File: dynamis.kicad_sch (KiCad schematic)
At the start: 201 parts, among them J0 USB_C_Receptacle_USB2.0, SW00_00 SW_Push, SW00_01 SW_Push, SW00_02 SW_Push, SW00_03 SW_Push, SW00_04 SW_Push, SW00_05 SW_Push, SW00_06 SW_Push, SW01_00 SW_Push, SW01_01 SW_Push, SW01_02 SW_Push, SW01_03 SW_Push, SW01_04 SW_Push, SW01_05 SW_Push, SW01_06 SW_Push, SW02_01 SW_Push, SW02_02 SW_Push, SW02_03 SW_Push, SW02_04 SW_Push, SW02_05 SW_Push, SW02_06 SW_Push, SW03_00 SW_Push, SW03_02 SW_Push, SW03_03 SW_Push, SW03_04 SW_Push, SW03_05 SW_Push, SW03_06 SW_Push, SW04_00 SW_Push, SW04_01 SW_Push, SW04_02 SW_Push, SW04_03 SW_Push, SW04_05 SW_Push, SW04_06 SW_Push, SW05_01 SW_Push, SW05_02 SW_Push, SW05_03 SW_Push, SW05_04 SW_Push, SW05_05 SW_Push, SW05_06 SW_Push, SW06_00 SW_Push, SW06_01 SW_Push, SW06_02 SW_Push, SW06_03 SW_Push, SW06_04 SW_Push, SW06_05 SW_Push, SW06_06 SW_Push, SW07_01 SW_Push, SW07_02 SW_Push, SW07_03 SW_Push, SW07_04 SW_Push, SW07_05 SW_Push, SW07_06 SW_Push, SW08_00 SW_Push, SW08_02 SW_Push, SW08_03 SW_Push, SW08_04 SW_Push, SW08_05 SW_Push, SW08_06 SW_Push, SW09_00 SW_Push, SW09_01 SW_Push, SW09_02 SW_Push, SW09_03 SW_Push, SW09_04 SW_Push, SW09_05 SW_Push, SW09_06 SW_Push, U0 ATmega32U4-M, U1 PMW3360DM-T2QU, U2 TPS73601DBV, U3 TPS73601DBV, U4 TPD4E05U06DQAR, Y0 16Mhz

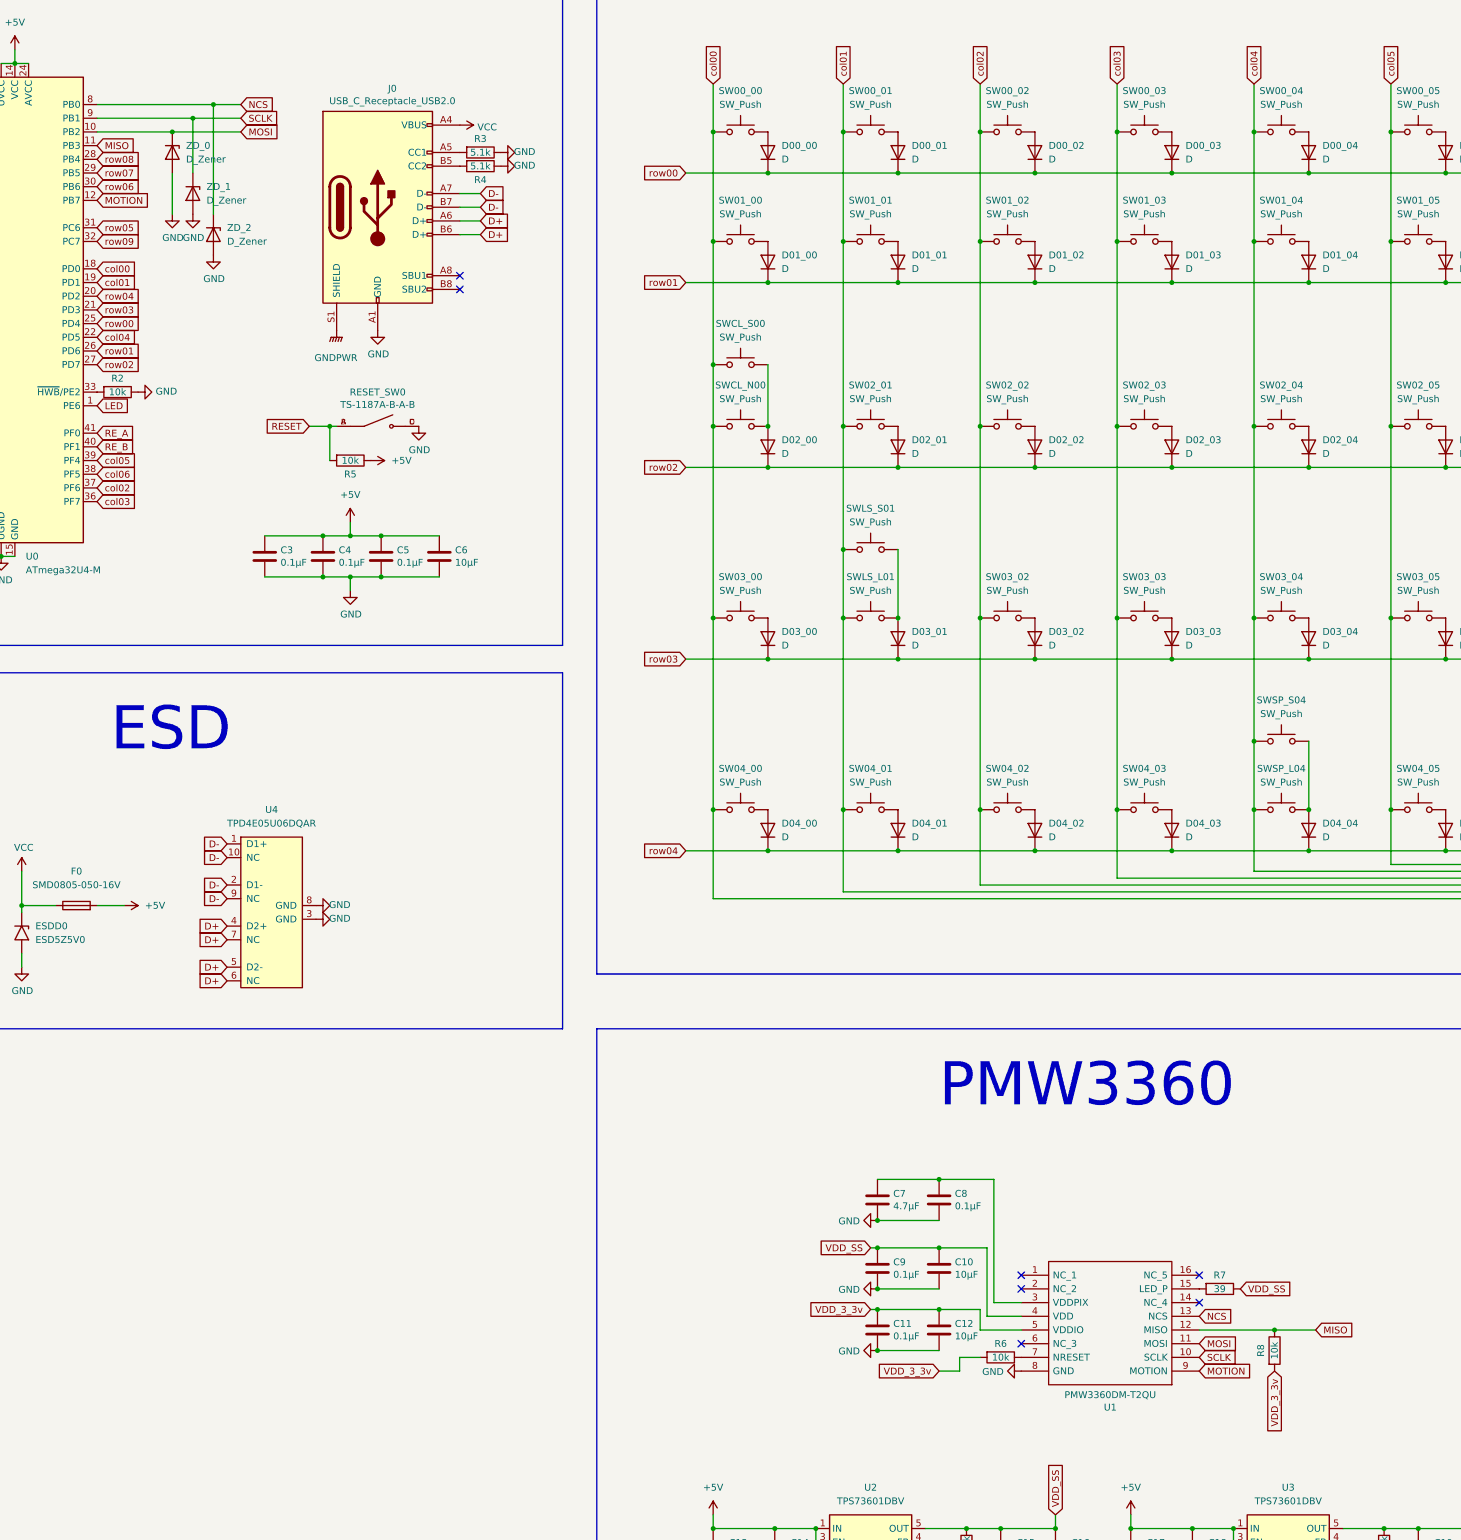
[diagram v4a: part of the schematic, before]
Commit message: dynamis v2
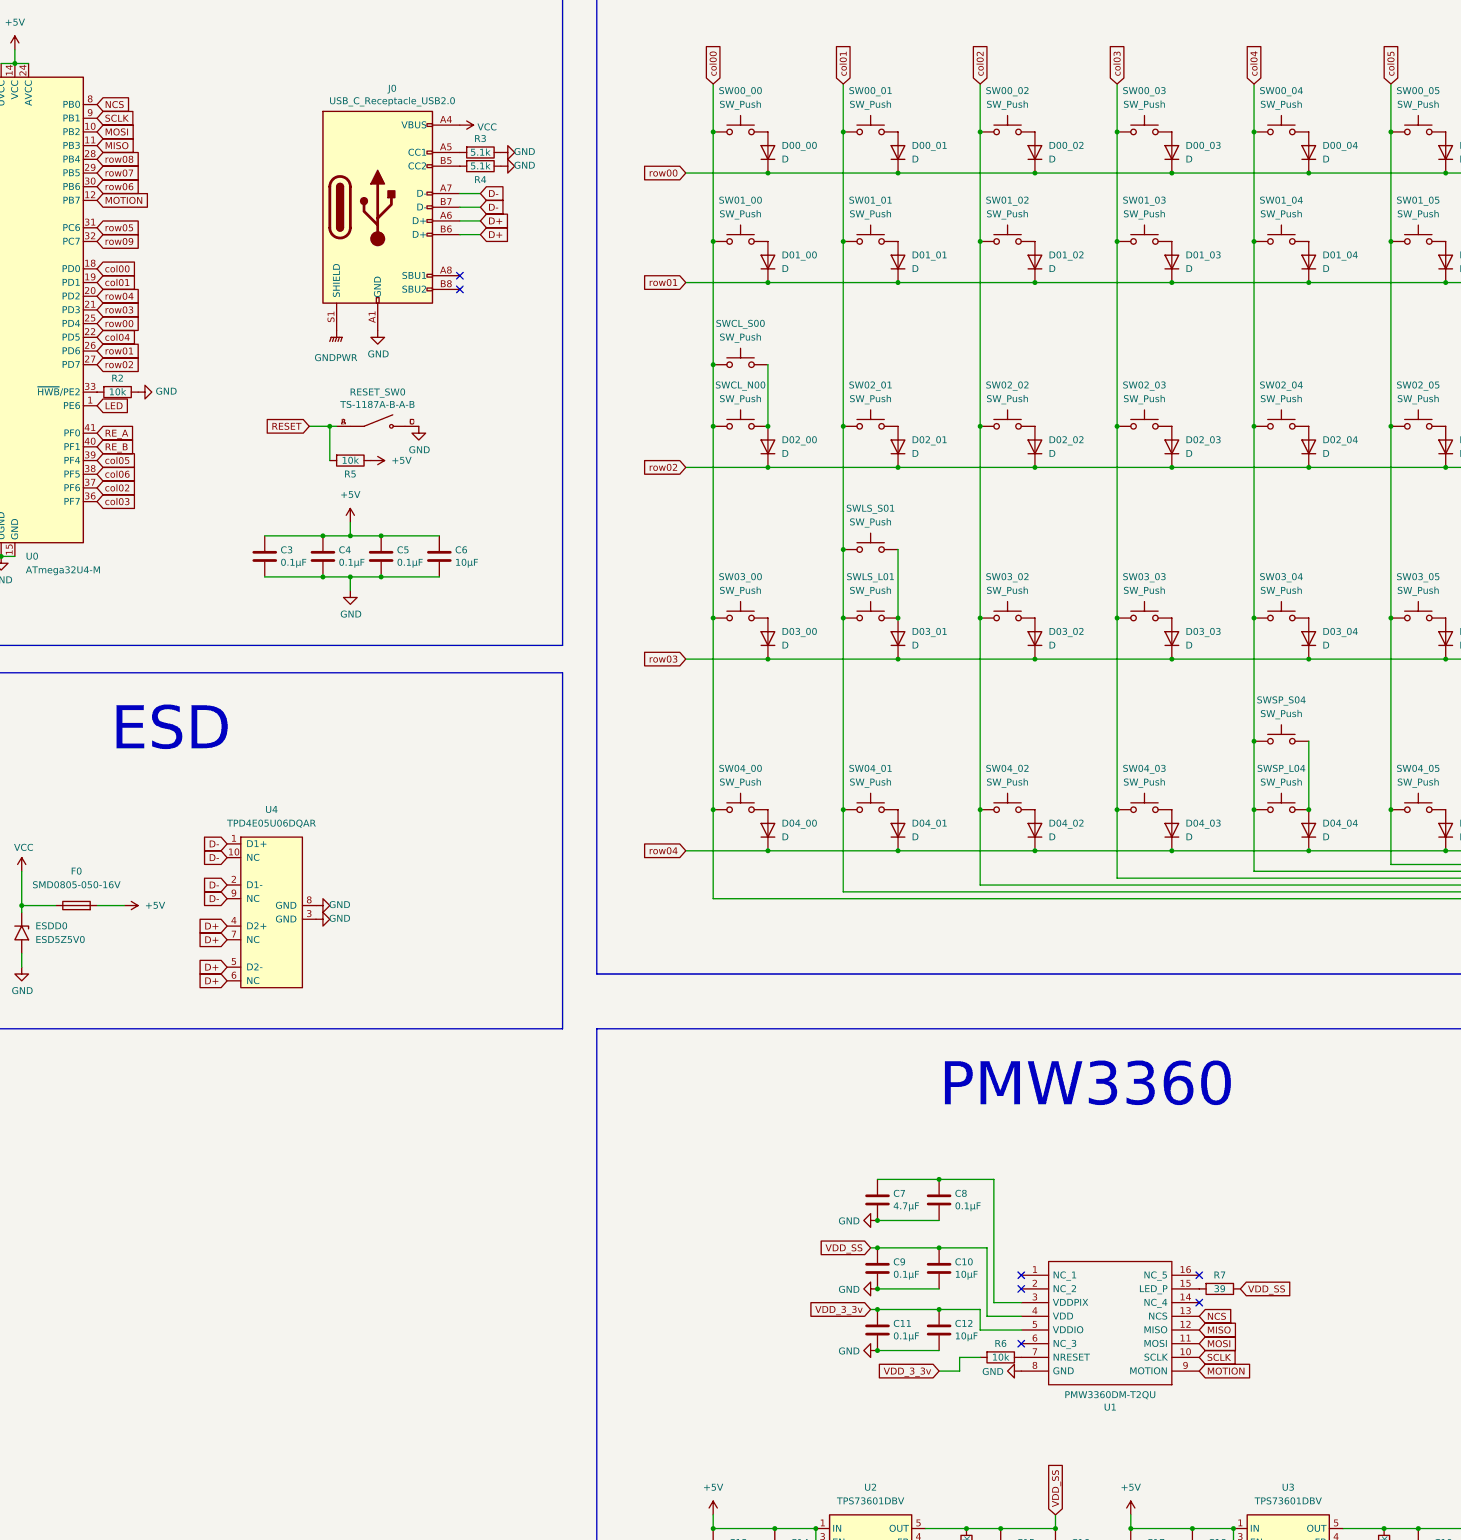
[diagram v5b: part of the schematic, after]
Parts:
- removed R8: 10k, Resistor_SMD:R_1206_3216Metric, symbol Device:R
- removed ZD_0, ZD_1, ZD_2: D_Zener, BZT52C3V3S:SOD-323_L1.6-W1.3-LS2.6-RD-1, symbol Device:D_Zener
